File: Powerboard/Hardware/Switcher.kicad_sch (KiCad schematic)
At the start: 40 parts, among them J1 Conn_01x03_MountingPin, J2 XT60PW-F, J7 XT60PW-M, J8 Conn_01x04_Male, U2 ESP32-S3, Y1 40MHz±10ppm

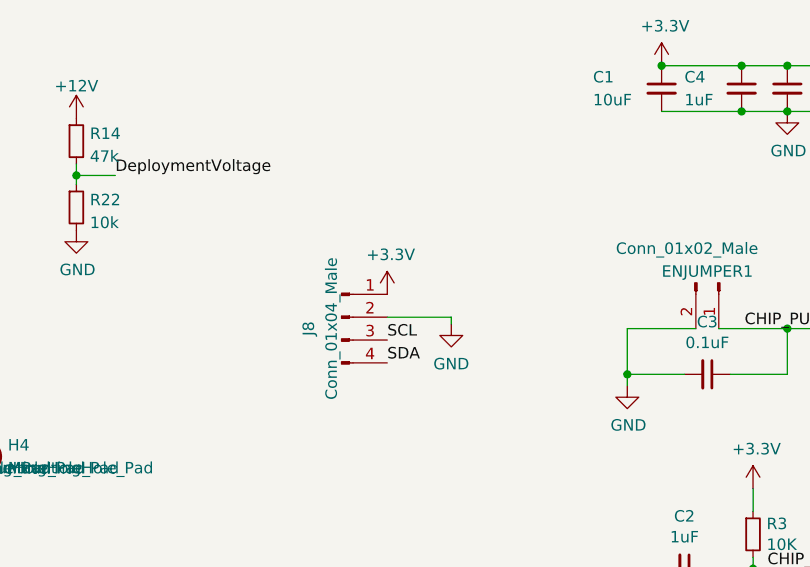
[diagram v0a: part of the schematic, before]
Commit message: kiran/andrei review
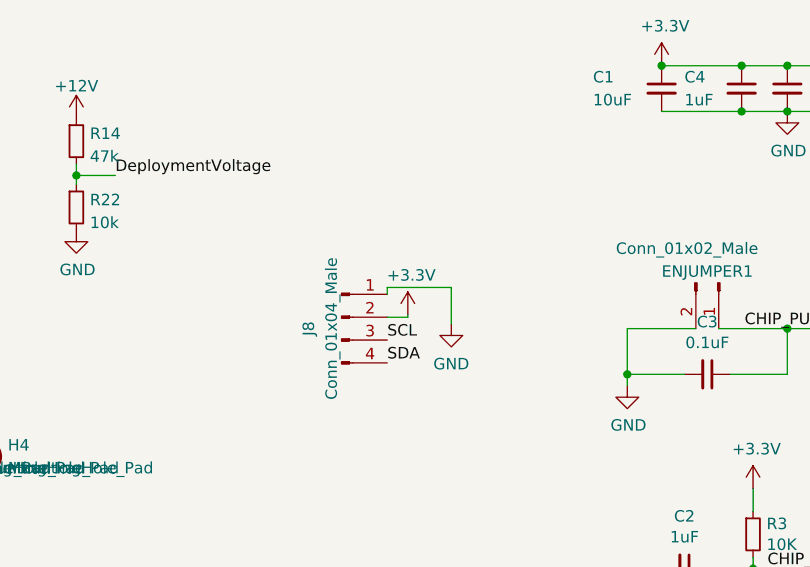
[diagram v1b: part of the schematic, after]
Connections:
- net +3V3: now also J8.2 (Pin_2); no longer J8.1 (Pin_1)
- net GND: now also J8.1 (Pin_1); no longer J8.2 (Pin_2)
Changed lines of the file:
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@@
+    (stroke (width 0) (type default))
+  )
+  (wire (pts (xy 96.012 164.592) (xy 98.298 164.592))
     (stroke (width 0) (type default))
   )
@@
     (stroke (width 0) (type default))
   )
+  (wire (pts (xy 96.012 161.29) (xy 96.012 162.052))
+    (stroke (width 0) (type default))
+  )
   (wire (pts (xy 126.492 141.732) (xy 135.382 141.732))
     (stroke (width 0) (type default))
@@
     (stroke (width 0) (type default))
   )
-  (wire (pts (xy 96.012 164.592) (xy 103.124 164.592))
-    (stroke (width 0) (type default))
-  )
   (wire (pts (xy 123.952 31.242) (xy 129.032 31.242))
     (stroke (width 0) (type default))
@@
     (stroke (width 0) (type default))
   )
-  (wire (pts (xy 103.124 164.592) (xy 103.124 165.354))
+  (wire (pts (xy 103.124 161.29) (xy 103.124 165.354))
     (stroke (width 0) (type default))
   )
@@
     (stroke (width 0) (type default))
   )
+  (wire (pts (xy 103.124 161.29) (xy 96.012 161.29))
+    (stroke (width 0) (type default))
+  )
   (wire (pts (xy 151.892 170.942) (xy 151.892 172.212))
     (stroke (width 0) (type default))
@@
   )
   (polyline (pts (xy 230.632 112.522) (xy 230.632 115.062))
+    (stroke (width 0) (type default))
+  )
+  (wire (pts (xy 98.298 164.592) (xy 98.298 164.338))
     (stroke (width 0) (type default))
   )
@@
     )
   )
-  (symbol (lib_id "power:+3.3V") (at 96.012 162.052 0) (unit 1)
-    (in_bom yes) (on_board yes) (dnp no)
-    (property "Reference" "#PWR0155" (at 96.012 165.862 0)
-      (effects (font (size 1.27 1.27)) hide)
-    )
-    (property "Value" "+3.3V" (at 96.393 157.6578 0)
-      (effects (font (size 1.27 1.27)))
-    )
-    (property "Footprint" "" (at 96.012 162.052 0)
-      (effects (font (size 1.27 1.27)) hide)
-    )
-    (property "Datasheet" "" (at 96.012 162.052 0)
-      (effects (font (size 1.27 1.27)) hide)
-    )
+  (symbol (lib_id "power:+3.3V") (at 98.298 164.338 0) (unit 1)
+    (in_bom yes) (on_board yes) (dnp no)
+    (property "Reference" "#PWR0155" (at 98.298 168.148 0)
+      (effects (font (size 1.27 1.27)) hide)
+    )
+    (property "Value" "+3.3V" (at 98.679 159.9438 0)
+      (effects (font (size 1.27 1.27)))
+    )
+    (property "Footprint" "" (at 98.298 164.338 0)
+      (effects (font (size 1.27 1.27)) hide)
+    )
+    (property "Datasheet" "" (at 98.298 164.338 0)
+      (effects (font (size 1.27 1.27)) hide)
+    )
